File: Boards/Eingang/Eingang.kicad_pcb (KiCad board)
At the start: 2 copper layers, 100 x 40 mm, 10 parts, among them P1 CONN_01X02, P2 CONN_01X02, P3 CONN_01X02, P4 CONN_01X03, P5 CONN_01X03, P6 CONN_01X03, P7 CONN_01X02, P8 CONN_01X02, P9 CONN_01X02

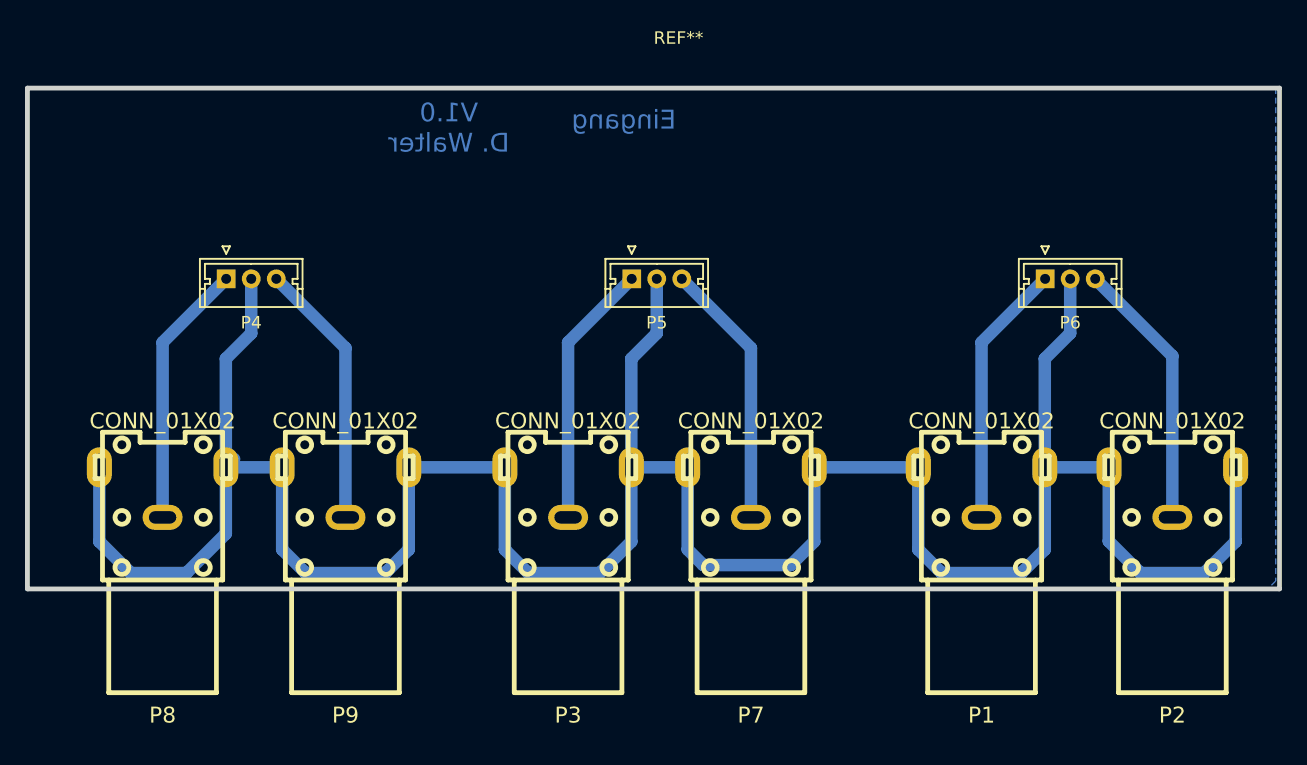
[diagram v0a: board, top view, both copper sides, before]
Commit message: Work in Progress
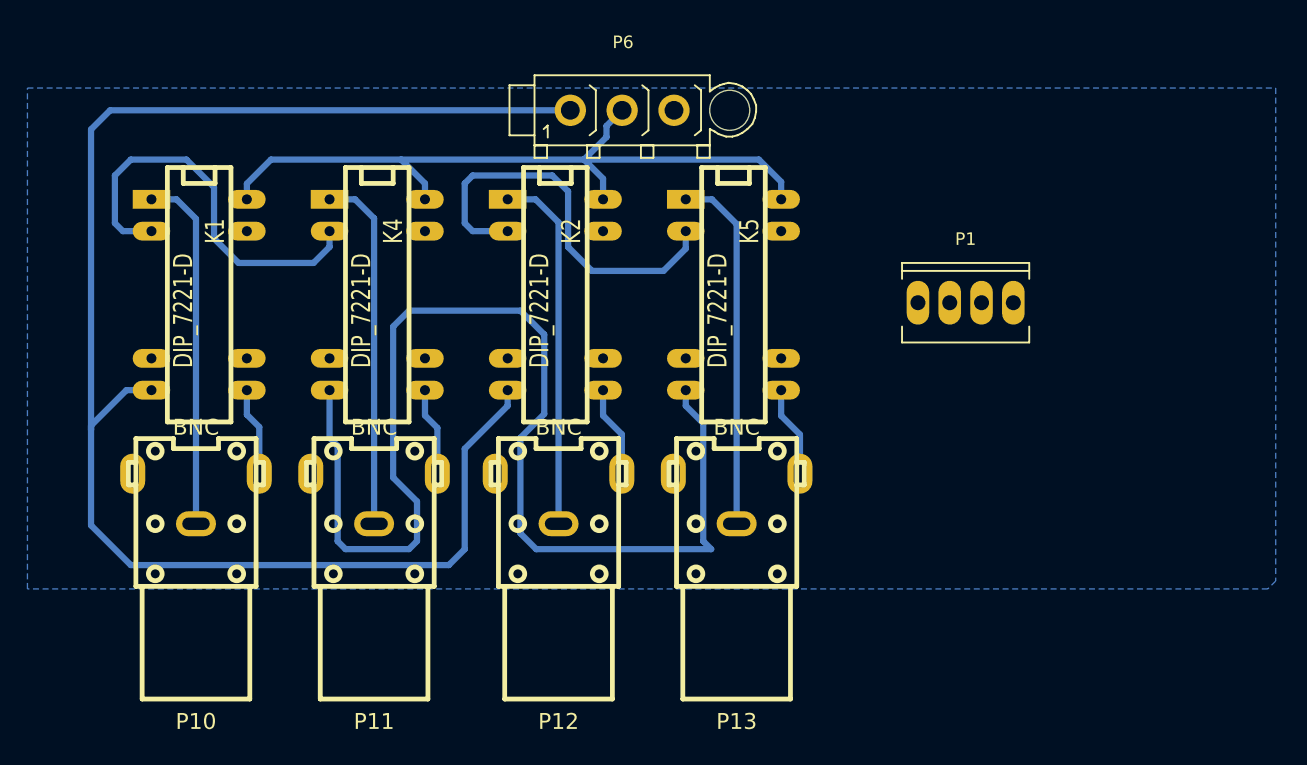
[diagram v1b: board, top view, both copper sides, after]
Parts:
- removed P2, P7, P9: CONN_01X02, w_conn_av:rca_red
- removed P3, P8: CONN_01X02, w_conn_av:rca_black
- removed P4, P5: CONN_01X03, Connectors_Molex:Molex_MicroLatch-53253-0370_03x2.00mm_Straight
- removed REF**: EuroBoard_viertel_Type-II_100mmX40mm, EuroBoard_Outline:EuroBoard_viertel_Type-II_100mmX40mm
- added K1: DIP_7221-D, Reed:REED, F.Cu at (103.9, 94.0)
- added K2: DIP_7221-D, Reed:REED, F.Cu at (132.3, 94.0)
- added K4: DIP_7221-D, Reed:REED, F.Cu at (118.1, 94.0)
- added K5: DIP_7221-D, Reed:REED, F.Cu at (146.6, 94.0)
- added P10: BNC, w_conn_av:rca_red, F.Cu at (103.6, 112.3)
- added P11: BNC, w_conn_av:rca_white, F.Cu at (117.9, 112.3)
- added P12: BNC, w_conn_av:rca_red, F.Cu at (132.6, 112.3)
- added P13: BNC, w_conn_av:rca_white, F.Cu at (146.8, 112.3)
- P1: value CONN_01X02 -> CONN_01X04; footprint w_conn_av:rca_black -> Sockets_MOLEX_KK-System:Socket_MOLEX-KK-RM2-54mm_Lock_4pin_straight
- P6: footprint Connectors_Molex:Molex_MicroLatch-53253-0370_03x2.00mm_Straight -> Sockets_Mini-Universal:MiniUniversalMate-N-LokSocket_3PinVertical
- moved P6 36.4 mm to (137.7, 79.2)
- moved P1 17.2 mm to (165.1, 94.6)
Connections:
- P1 pad 1: Net-(P1-Pad1) -> Net-(K1-Pad2)
- P1 pad 2: Earth_Clean -> Net-(K2-Pad2)
- P6 pad 1: Net-(P1-Pad1) -> Net-(K1-Pad7)
- P6 pad 2: Earth_Clean -> Net-(K1-Pad14)
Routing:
- net Earth_Clean: track 224.4 -> 0.00 mm
- net Net-(K1-Pad7): track 0.00 -> 122.7 mm
- net Net-(K4-Pad7): track 21.6 -> 96.5 mm
- net Net-(K1-Pad14): track 0.00 -> 59.8 mm
- net Net-(K2-Pad2): track 0.00 -> 33.4 mm
- net Net-(K1-Pad2): track 0.00 -> 32.3 mm
- net Net-(K2-Pad1): track 0.00 -> 28.9 mm
- net Net-(K5-Pad1): track 0.00 -> 28.8 mm
- net Net-(K4-Pad1): track 0.00 -> 28.6 mm
- net Net-(K1-Pad1): track 0.00 -> 28.6 mm
- net Net-(P5-Pad3): track 21.3 -> 0.00 mm
- net Net-(P4-Pad3): track 21.3 -> 0.00 mm
- net Net-(P3-Pad1): track 21.2 -> 0.00 mm
- net Net-(P4-Pad1): track 21.2 -> 0.00 mm
- net Net-(P1-Pad1): track 21.2 -> 0.00 mm
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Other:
- board outline removed
- board text removed: "Eingang"
- board text removed: "V1.0 D. Walter"

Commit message: Work in Progress
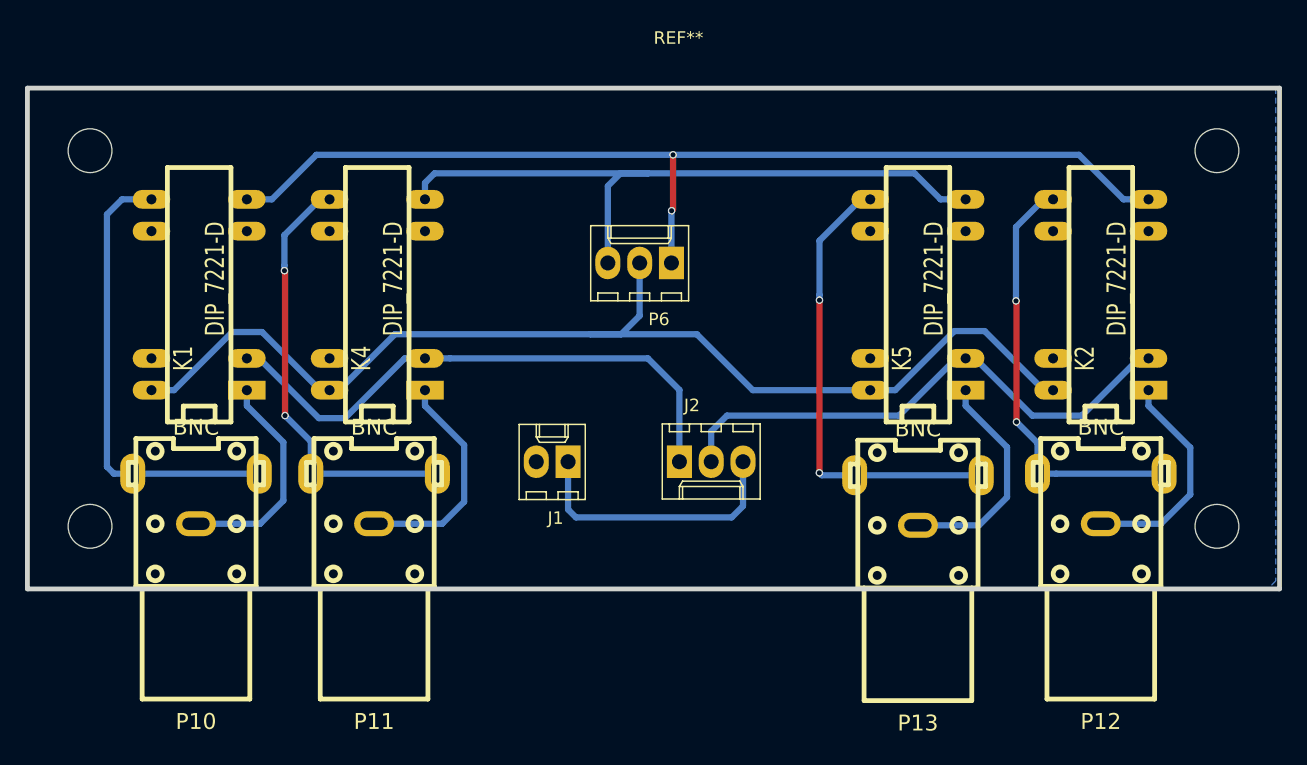
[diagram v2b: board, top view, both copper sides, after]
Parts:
- removed P1: CONN_01X04, Sockets_MOLEX_KK-System:Socket_MOLEX-KK-RM2-54mm_Lock_4pin_straight
- added J1: Conn_01x02, Connectors_Molex:Molex_KK-6410-02_02x2.54mm_Straight, F.Cu at (133.3, 107.3)
- added J2: Conn_01x03, Connectors_Molex:Molex_KK-6410-03_03x2.54mm_Straight, F.Cu at (142.2, 107.3)
- added REF**: EuroBoard_viertel_Type-II_100mmX40mm_holes, EuroBoard_Outline:EuroBoard_viertel_Type-II_100mmX40mm_holes, F.Cu at (90.2, 117.5)
- P6: footprint Sockets_Mini-Universal:MiniUniversalMate-N-LokSocket_3PinVertical -> Connectors_Molex:Molex_KK-6410-03_03x2.54mm_Straight
- moved K2 43.6 mm to (175.9, 94.0), turned to 90 degrees
- moved P12 43.3 mm to (175.9, 112.3)
- moved K5 14.7 mm to (161.3, 94.0), turned to 90 degrees
- moved P13 14.5 mm to (161.3, 112.4)
- moved P6 12.8 mm to (141.6, 91.4), turned to 180 degrees
- turned K1 to 90 degrees
- turned K4 to 90 degrees
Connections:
- net Net-(K1-Pad6) renamed GND
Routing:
- net Net-(K4-Pad7): track 96.5 -> 56.2 mm
- net Net-(K1-Pad7): track 122.7 -> 84.4 mm, vias 0 -> 2
- net Net-(K1-Pad14): track 59.8 -> 92.2 mm
- net Net-(K5-Pad8): track 7.29 -> 37.0 mm, vias 0 -> 2
- net Net-(K1-Pad8): track 7.08 -> 36.6 mm
- net Net-(K4-Pad8): track 7.08 -> 34.8 mm, vias 0 -> 2
- net Net-(K2-Pad8): track 7.29 -> 34.4 mm, vias 0 -> 2
- net Net-(J1-Pad1): track 0.00 -> 22.0 mm
- net Net-(J2-Pad1): track 32.3 -> 45.3 mm
- net Net-(K2-Pad1): track 28.9 -> 17.8 mm
- net Net-(K5-Pad1): track 28.8 -> 18.0 mm
- net Net-(K1-Pad1): track 28.6 -> 17.8 mm
- net Net-(K4-Pad1): track 28.6 -> 18.1 mm
- net Net-(J2-Pad2): track 33.4 -> 43.6 mm
- added copper zone on B.Cu, net GND
- removed copper zone on B.Cu, net Earth_Clean
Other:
- board outline added: 100 x 40 mm
